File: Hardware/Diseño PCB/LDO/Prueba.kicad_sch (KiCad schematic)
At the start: 54 parts, among them Q1 2N3904, Q10 BC557, Q11 BC547, Q12 BC557, Q13 2N3906, Q14 2N3904, Q15 2N3906, Q16 2N3904, Q17 2N3906, Q18 2N3904, Q19 2N3904, Q2 2N3904, Q3 2N3904, Q4 2N3906, Q5 2N3906, Q6 2N3904, Q7 2N3904, Q8 IRF4905, Q9 BC547, U1 TL431LP, U4 LM324

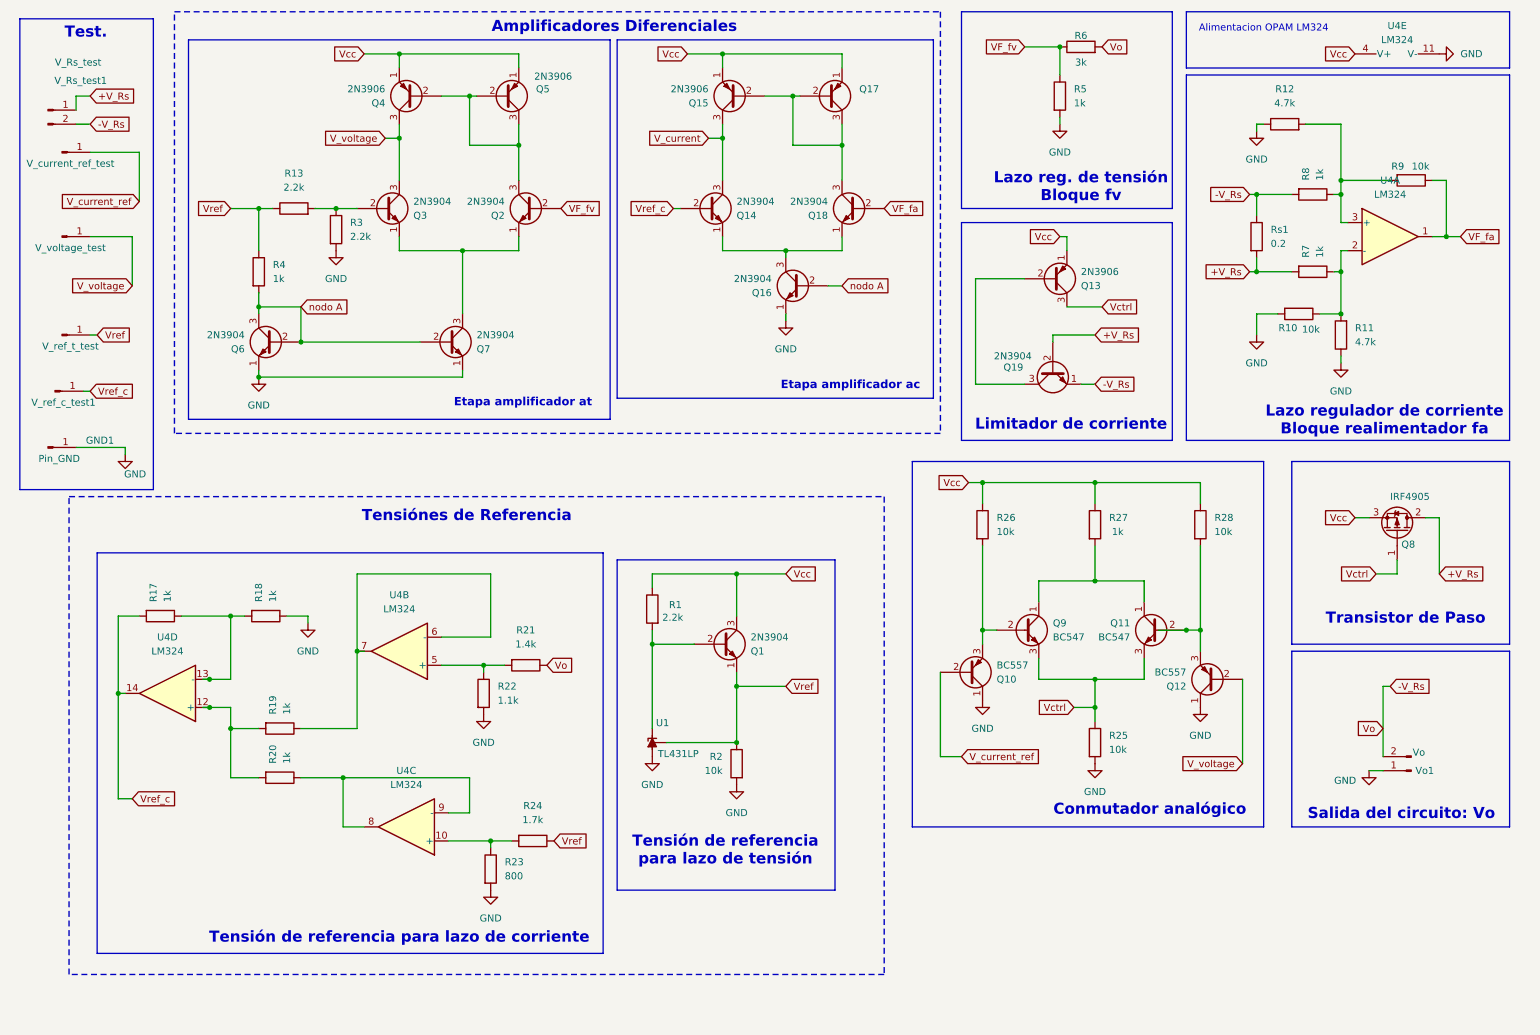
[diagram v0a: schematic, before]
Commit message: PCB: Diseño
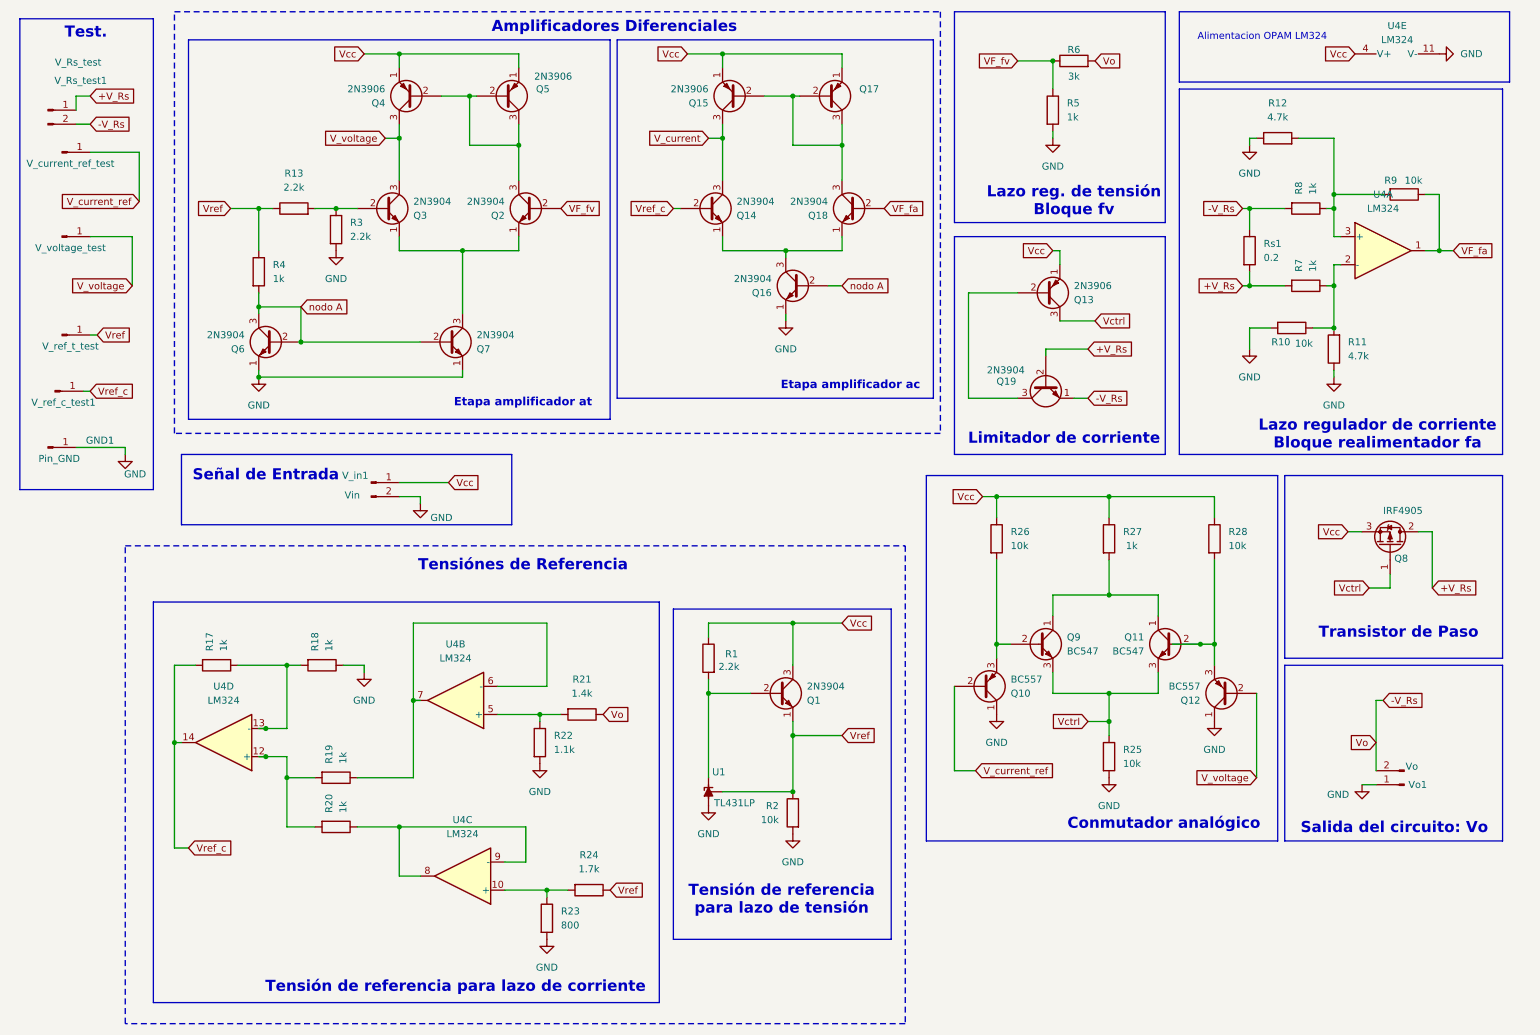
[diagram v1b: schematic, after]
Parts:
- added V_in1: Vin, Connector_PinHeader_2.00mm:PinHeader_1x02_P2.00mm_Vertical, symbol Connector:Conn_01x02_Pin
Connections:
- net GND: now also V_in1.2 (Pin_2)
- net Vcc: now also V_in1.1 (Pin_1)
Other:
- note added: "Señal de Entrada"
- moved on the sheet: Q1, Q10, Q11, Q12, Q13, Q19, Q8, Q9, R1, R10, R11, R12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
